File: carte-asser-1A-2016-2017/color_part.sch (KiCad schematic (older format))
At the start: 16 parts, among them P22 CONN_01X02, P23 CONN_01X02, P24 CONN_01X02, U10 OP275, U11 OP275

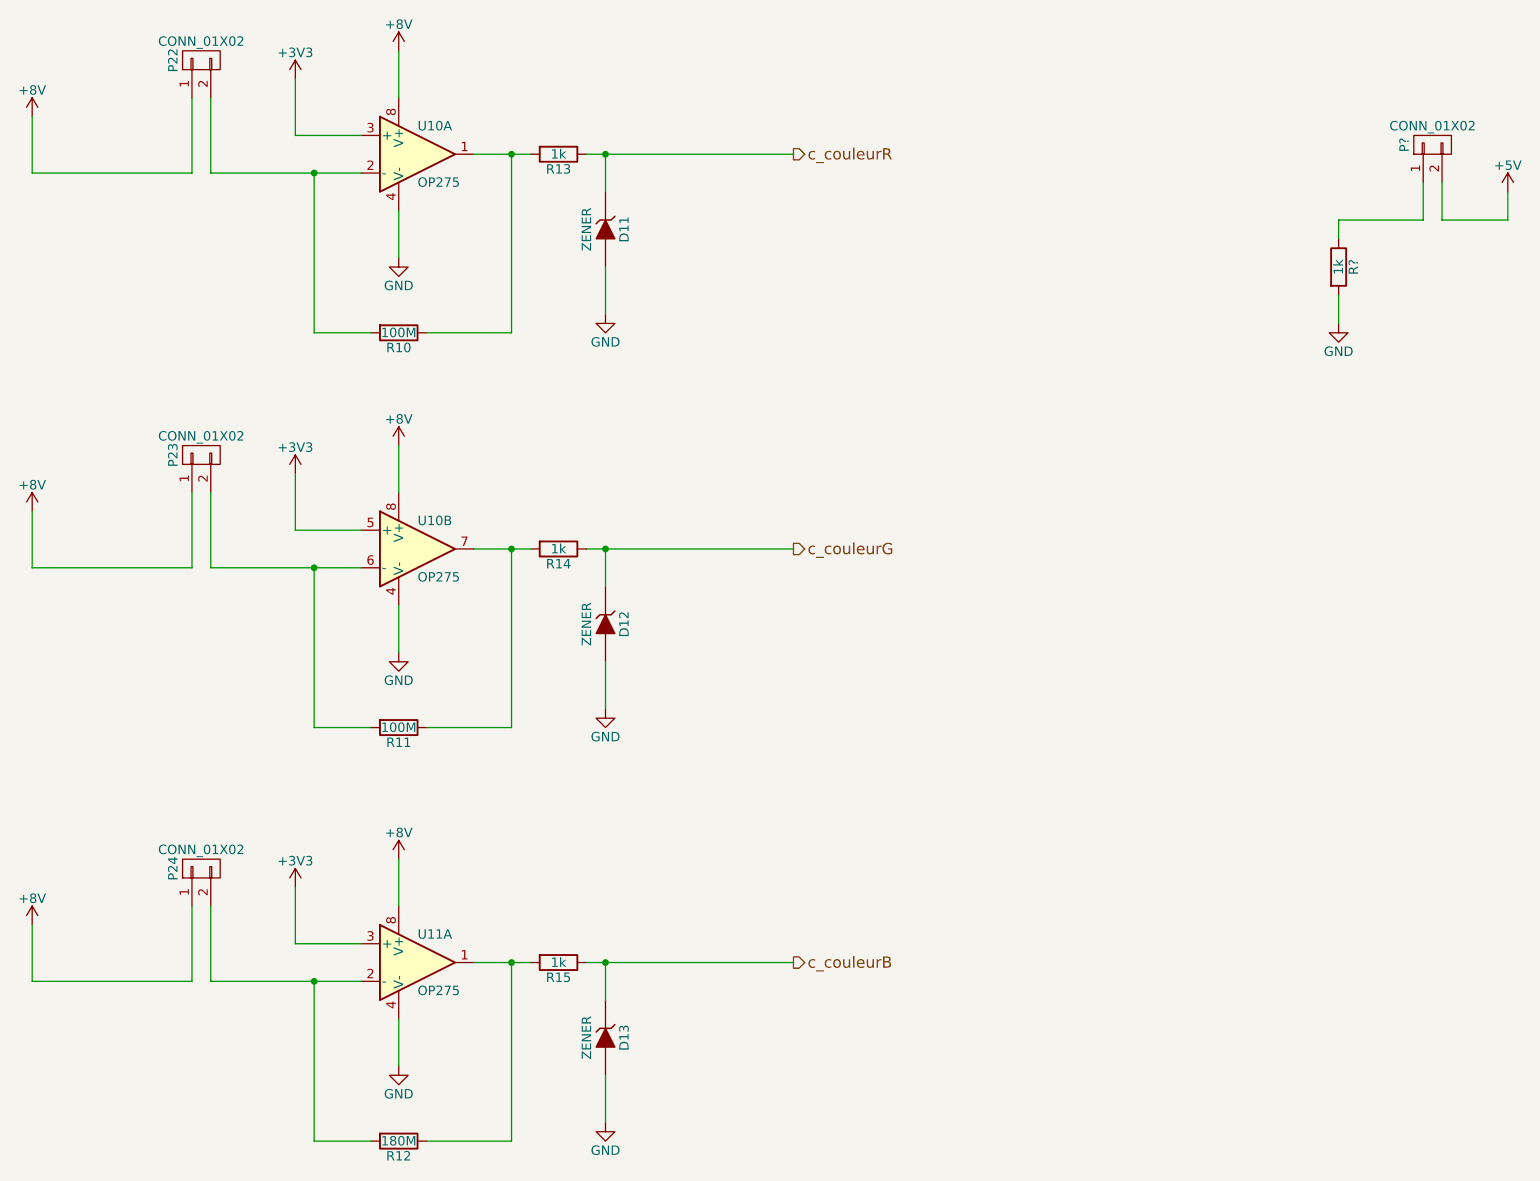
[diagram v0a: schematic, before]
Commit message: PCB
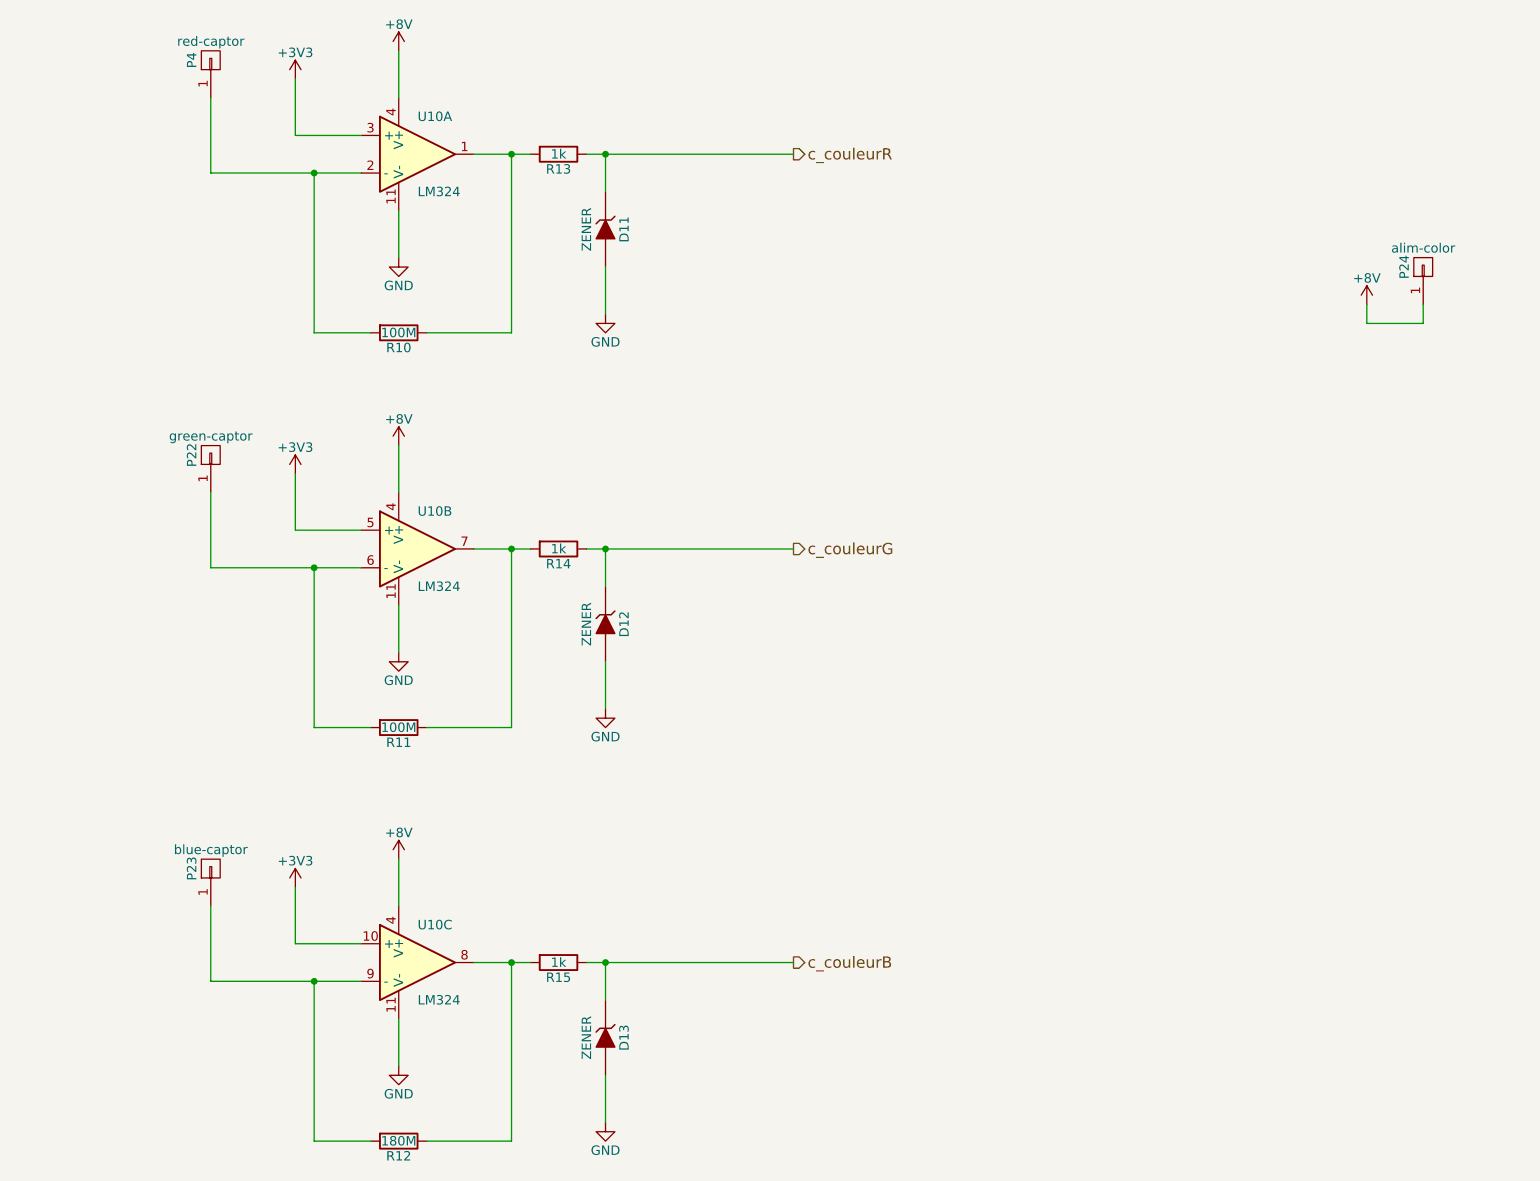
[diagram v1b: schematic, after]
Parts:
- removed P22, P23, P24, P?: CONN_01X02, symbol CONN_01X02
- removed R?: 1k, symbol R
- removed U10, U11: OP275, symbol OP275
- added P22: green-captor, Pin_Headers:Pin_Header_Straight_1x01_Pitch2.54mm, symbol CONN_01X01
- added P23: blue-captor, Pin_Headers:Pin_Header_Straight_1x01_Pitch2.54mm, symbol CONN_01X01
- added P24: alim-color, Pin_Headers:Pin_Header_Straight_1x01_Pitch2.54mm, symbol CONN_01X01
- added P4: red-captor, Pin_Headers:Pin_Header_Straight_1x01_Pitch2.54mm, symbol CONN_01X01
- added U10: LM324, Housings_DIP:DIP-16_W7.62mm, symbol LM324
- D11, D12, D13, R10, R11, R12, R13, R14, R15: footprint (none) -> Discret:R4-LARGE_PADS
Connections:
- net +3V3: now also U10.10 (+), U10.3 (+), U10.5 (+)
- net +8V: now also P24.1 (P1), U10.4 (V+), U10.4 (V+), U10.4 (V+)
- net GND: now also U10.11 (V-), U10.11 (V-), U10.11 (V-)
- net at R10.2: now also P4.1 (P1), U10.2 (-)
- net at R10.1, R13.2: now also U10.1
- net at R11.2: now also P22.1 (P1), U10.6 (-)
- net at R11.1, R14.2: now also U10.7
- net at R12.2: now also P23.1 (P1), U10.9 (-)
- net at R12.1, R15.2: now also U10.8
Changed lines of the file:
@@
 $Descr A4 11693 8268
 encoding utf-8
-Sheet 6 8
+Sheet 6 9
 Title ""
 Date ""
@@
 Comment4 ""
 $EndDescr
-$Comp
-L CONN_01X02 P22
-U 1 1 58A6B5A3
-P 2800 1250
-F 0 "P22" H 2800 1400 50  0000 C CNN
-F 1 "CONN_01X02" V 2900 1250 50  0000 C CNN
-F 2 "" H 2800 1250 50  0000 C CNN
-F 3 "" H 2800 1250 50  0000 C CNN
-	1    2800 1250
-	0    -1   -1   0
-$EndComp
-Wire Wire Line
-	2750 1450 2750 1850
-Wire Wire Line
-	2750 1850 1900 1850
 Wire Wire Line
 	2850 1450 2850 1850
 Wire Wire Line
 	2850 1850 3650 1850
-$Comp
-L OP275 U10
-U 1 1 58A6B640
-P 3950 1750
-F 0 "U10" H 3950 1900 50  0000 L CNN
-F 1 "OP275" H 3950 1600 50  0000 L CNN
-F 2 "" H 3850 1800 50  0000 C CNN
-F 3 "" H 3950 1900 50  0000 C CNN
-	1    3950 1750
-	1    0    0    -1
-$EndComp
 Wire Wire Line
 	3400 1850 3400 2700
@@
 F 0 "R10" V 3930 2700 50  0000 C CNN
 F 1 "100M" V 3850 2700 50  0000 C CNN
-F 2 "" V 3780 2700 50  0000 C CNN
+F 2 "Discret:R4-LARGE_PADS" V 3780 2700 50  0001 C CNN
 F 3 "" H 3850 2700 50  0000 C CNN
 	1    3850 2700
@@
 F 0 "D11" H 4950 2250 50  0000 C CNN
 F 1 "ZENER" H 4950 2050 50  0000 C CNN
-F 2 "" H 4950 2150 50  0000 C CNN
+F 2 "Discret:R4-LARGE_PADS" H 4950 2150 50  0001 C CNN
 F 3 "" H 4950 2150 50  0000 C CNN
 	1    4950 2150
@@
 	3850 1450 3850 1200
 Wire Wire Line
-	1900 1850 1900 1550
-$Comp
-L CONN_01X02 P23
-U 1 1 58A72BC5
-P 2800 3350
-F 0 "P23" H 2800 3500 50  0000 C CNN
-F 1 "CONN_01X02" V 2900 3350 50  0000 C CNN
-F 2 "" H 2800 3350 50  0000 C CNN
-F 3 "" H 2800 3350 50  0000 C CNN
-	1    2800 3350
-	0    -1   -1   0
-$EndComp
-Wire Wire Line
-	2750 3550 2750 3950
-Wire Wire Line
-	2750 3950 1900 3950
-Wire Wire Line
 	2850 3550 2850 3950
 Wire Wire Line
 	2850 3950 3650 3950
-$Comp
-L OP275 U10
-U 2 1 58A72BCF
-P 3950 3850
-F 0 "U10" H 3950 4000 50  0000 L CNN
-F 1 "OP275" H 3950 3700 50  0000 L CNN
-F 2 "" H 3850 3900 50  0000 C CNN
-F 3 "" H 3950 4000 50  0000 C CNN
-	2    3950 3850
-	1    0    0    -1
-$EndComp
 Wire Wire Line
 	3400 3950 3400 4800
@@
 F 0 "R11" V 3930 4800 50  0000 C CNN
 F 1 "100M" V 3850 4800 50  0000 C CNN
-F 2 "" V 3780 4800 50  0000 C CNN
+F 2 "Discret:R4-LARGE_PADS" V 3780 4800 50  0001 C CNN
 F 3 "" H 3850 4800 50  0000 C CNN
 	1    3850 4800
@@
 F 0 "D12" H 4950 4350 50  0000 C CNN
 F 1 "ZENER" H 4950 4150 50  0000 C CNN
-F 2 "" H 4950 4250 50  0000 C CNN
+F 2 "Discret:R4-LARGE_PADS" H 4950 4250 50  0001 C CNN
 F 3 "" H 4950 4250 50  0000 C CNN
 	1    4950 4250
@@
 	3850 3550 3850 3300
 Wire Wire Line
-	1900 3950 1900 3650
-$Comp
-L CONN_01X02 P24
-U 1 1 58A72E17
-P 2800 5550
-F 0 "P24" H 2800 5700 50  0000 C CNN
-F 1 "CONN_01X02" V 2900 5550 50  0000 C CNN
-F 2 "" H 2800 5550 50  0000 C CNN
-F 3 "" H 2800 5550 50  0000 C CNN
-	1    2800 5550
-	0    -1   -1   0
-$EndComp
-Wire Wire Line
-	2750 5750 2750 6150
-Wire Wire Line
-	2750 6150 1900 6150
-Wire Wire Line
 	2850 5750 2850 6150
 Wire Wire Line
 	2850 6150 3650 6150
-$Comp
-L OP275 U11
-U 1 1 58A72E21
-P 3950 6050
-F 0 "U11" H 3950 6200 50  0000 L CNN
-F 1 "OP275" H 3950 5900 50  0000 L CNN
-F 2 "" H 3850 6100 50  0000 C CNN
-F 3 "" H 3950 6200 50  0000 C CNN
-	1    3950 6050
-	1    0    0    -1
-$EndComp
 Wire Wire Line
 	3400 6150 3400 7000
@@
 F 0 "R12" V 3930 7000 50  0000 C CNN
 F 1 "180M" V 3850 7000 50  0000 C CNN
-F 2 "" V 3780 7000 50  0000 C CNN
+F 2 "Discret:R4-LARGE_PADS" V 3780 7000 50  0001 C CNN
 F 3 "" H 3850 7000 50  0000 C CNN
 	1    3850 7000
@@
 F 0 "D13" H 4950 6550 50  0000 C CNN
 F 1 "ZENER" H 4950 6350 50  0000 C CNN
-F 2 "" H 4950 6450 50  0000 C CNN
+F 2 "Discret:R4-LARGE_PADS" H 4950 6450 50  0001 C CNN
 F 3 "" H 4950 6450 50  0000 C CNN
 	1    4950 6450
@@
 Wire Wire Line
 	3850 5750 3850 5500
-Wire Wire Line
-	1900 6150 1900 5850
 $Comp
 L +8V #PWR061
@@
 L +8V #PWR062
 U 1 1 58A7EE3E
-P 1900 1550
-F 0 "#PWR062" H 1900 1400 50  0001 C CNN
-F 1 "+8V" H 1900 1690 50  0000 C CNN
-F 2 "" H 1900 1550 50  0000 C CNN
-F 3 "" H 1900 1550 50  0000 C CNN
-	1    1900 1550
+P 9000 2550
+F 0 "#PWR062" H 9000 2400 50  0001 C CNN
+F 1 "+8V" H 9000 2690 50  0000 C CNN
+F 2 "" H 9000 2550 50  0000 C CNN
+F 3 "" H 9000 2550 50  0000 C CNN
+	1    9000 2550
 	1    0    0    -1
 $EndComp
 $Comp
 L +8V #PWR063
-U 1 1 58A7EF37
-P 1900 3650
-F 0 "#PWR063" H 1900 3500 50  0001 C CNN
-F 1 "+8V" H 1900 3790 50  0000 C CNN
-F 2 "" H 1900 3650 50  0000 C CNN
-F 3 "" H 1900 3650 50  0000 C CNN
-	1    1900 3650
-	1    0    0    -1
-$EndComp
-$Comp
-L +8V #PWR064
 U 1 1 58A7EFDC
 P 3850 3300
-F 0 "#PWR064" H 3850 3150 50  0001 C CNN
+F 0 "#PWR063" H 3850 3150 50  0001 C CNN
 F 1 "+8V" H 3850 3440 50  0000 C CNN
 F 2 "" H 3850 3300 50  0000 C CNN
@@
 $EndComp
 $Comp
-L +8V #PWR065
-U 1 1 58A7F1A1
-P 1900 5850
-F 0 "#PWR065" H 1900 5700 50  0001 C CNN
-F 1 "+8V" H 1900 5990 50  0000 C CNN
-F 2 "" H 1900 5850 50  0000 C CNN
-F 3 "" H 1900 5850 50  0000 C CNN
-	1    1900 5850
-	1    0    0    -1
-$EndComp
-$Comp
-L +8V #PWR066
+L +8V #PWR064
 U 1 1 58A7F216
 P 3850 5500
-F 0 "#PWR066" H 3850 5350 50  0001 C CNN
+F 0 "#PWR064" H 3850 5350 50  0001 C CNN
 F 1 "+8V" H 3850 5640 50  0000 C CNN
 F 2 "" H 3850 5500 50  0000 C CNN
@@
 $EndComp
 $Comp
-L +3V3 #PWR067
+L +3V3 #PWR065
 U 1 1 58A7F34D
 P 3300 5650
-F 0 "#PWR067" H 3300 5500 50  0001 C CNN
+F 0 "#PWR065" H 3300 5500 50  0001 C CNN
 F 1 "+3V3" H 3300 5790 50  0000 C CNN
 F 2 "" H 3300 5650 50  0000 C CNN
@@
 $EndComp
 $Comp
-L +3V3 #PWR068
+L +3V3 #PWR066
 U 1 1 58A7F40A
 P 3300 3450
-F 0 "#PWR068" H 3300 3300 50  0001 C CNN
+F 0 "#PWR066" H 3300 3300 50  0001 C CNN
 F 1 "+3V3" H 3300 3590 50  0000 C CNN
 F 2 "" H 3300 3450 50  0000 C CNN
@@
 $EndComp
 $Comp
-L +3V3 #PWR069
+L +3V3 #PWR067
 U 1 1 58A7F4D3
 P 3300 1350
-F 0 "#PWR069" H 3300 1200 50  0001 C CNN
+F 0 "#PWR067" H 3300 1200 50  0001 C CNN
 F 1 "+3V3" H 3300 1490 50  0000 C CNN
 F 2 "" H 3300 1350 50  0000 C CNN
@@
 F 0 "R13" V 4780 1750 50  0000 C CNN
 F 1 "1k" V 4700 1750 50  0000 C CNN
-F 2 "" V 4630 1750 50  0000 C CNN
+F 2 "Discret:R4-LARGE_PADS" V 4630 1750 50  0001 C CNN
 F 3 "" H 4700 1750 50  0000 C CNN
 	1    4700 1750
@@
 F 0 "R14" V 4780 3850 50  0000 C CNN
 F 1 "1k" V 4700 3850 50  0000 C CNN
-F 2 "" V 4630 3850 50  0000 C CNN
+F 2 "Discret:R4-LARGE_PADS" V 4630 3850 50  0001 C CNN
 F 3 "" H 4700 3850 50  0000 C CNN
 	1    4700 3850
@@
 F 0 "R15" V 4780 6050 50  0000 C CNN
 F 1 "1k" V 4700 6050 50  0000 C CNN
-F 2 "" V 4630 6050 50  0000 C CNN
+F 2 "Discret:R4-LARGE_PADS" V 4630 6050 50  0001 C CNN
 F 3 "" H 4700 6050 50  0000 C CNN
 	1    4700 6050
@@
 	4850 1750 5950 1750
 $Comp
-L CONN_01X02 P?
-U 1 1 58B3D98B
-P 9350 1700
-F 0 "P?" H 9350 1850 50  0000 C CNN
-F 1 "CONN_01X02" V 9450 1700 50  0000 C CNN
-F 2 "" H 9350 1700 50  0000 C CNN
-F 3 "" H 9350 1700 50  0000 C CNN
-	1    9350 1700
+L CONN_01X01 P4
+U 1 1 58BB9EC9
+P 2850 1250
+F 0 "P4" H 2850 1350 50  0000 C CNN
+F 1 "red-captor" V 2950 1250 50  0000 C CNN
+F 2 "Pin_Headers:Pin_Header_Straight_1x01_Pitch2.54mm" H 2850 1250 50  0001 C CNN
+F 3 "" H 2850 1250 50  0000 C CNN
+	1    2850 1250
 	0    -1   -1   0
 $EndComp
-Wire Wire Line
-	9300 1900 9300 2100
-Wire Wire Line
-	9300 2100 8850 2100
-Wire Wire Line
-	8850 2100 8850 2200
-$Comp
-L R R?
-U 1 1 58B3DB16
-P 8850 2350
-F 0 "R?" V 8930 2350 50  0000 C CNN
-F 1 "1k" V 8850 2350 50  0000 C CNN
-F 2 "" V 8780 2350 50  0000 C CNN
-F 3 "" H 8850 2350 50  0000 C CNN
-	1    8850 2350
-	1    0    0    -1
-$EndComp
-Wire Wire Line
-	8850 2500 8850 2650
-$Comp
-L GND #PWR070
-U 1 1 58B3DBAA
-P 8850 2650
-F 0 "#PWR070" H 8850 2400 50  0001 C CNN
-F 1 "GND" H 8850 2500 50  0000 C CNN
-F 2 "" H 8850 2650 50  0000 C CNN
-F 3 "" H 8850 2650 50  0000 C CNN
-	1    8850 2650
-	1    0    0    -1
-$EndComp
-Wire Wire Line
-	9400 1900 9400 2100
-Wire Wire Line
-	9400 2100 9750 2100
-Wire Wire Line
-	9750 2100 9750 1950
-$Comp
-L +5V #PWR071
-U 1 1 58B3DC7A
-P 9750 1950
-F 0 "#PWR071" H 9750 1800 50  0001 C CNN
-F 1 "+5V" H 9750 2090 50  0000 C CNN
-F 2 "" H 9750 1950 50  0000 C CNN
-F 3 "" H 9750 1950 50  0000 C CNN
-	1    9750 1950
-	1    0    0    -1
-$EndComp
+$Comp
+L CONN_01X01 P24
+U 1 1 58BB9FC6
+P 9300 2350
+F 0 "P24" H 9300 2450 50  0000 C CNN
+F 1 "alim-color" V 9400 2350 50  0000 C CNN
+F 2 "Pin_Headers:Pin_Header_Straight_1x01_Pitch2.54mm" H 9300 2350 50  0001 C CNN
+F 3 "" H 9300 2350 50  0000 C CNN
+	1    9300 2350
+	0    -1   -1   0
+$EndComp
+Wire Wire Line
+	9000 2650 9300 2650
+Wire Wire Line
+	9300 2650 9300 2550
+$Comp
+L CONN_01X01 P22
+U 1 1 58BBA20A
+P 2850 3350
+F 0 "P22" H 2850 3450 50  0000 C CNN
+F 1 "green-captor" V 2950 3350 50  0000 C CNN
+F 2 "Pin_Headers:Pin_Header_Straight_1x01_Pitch2.54mm" H 2850 3350 50  0001 C CNN
+F 3 "" H 2850 3350 50  0000 C CNN
+	1    2850 3350
+	0    -1   -1   0
+$EndComp
+$Comp
+L CONN_01X01 P23
+U 1 1 58BBA3AD
+P 2850 5550
+F 0 "P23" H 2850 5650 50  0000 C CNN
+F 1 "blue-captor" V 2950 5550 50  0000 C CNN
+F 2 "Pin_Headers:Pin_Header_Straight_1x01_Pitch2.54mm" H 2850 5550 50  0001 C CNN
+F 3 "" H 2850 5550 50  0000 C CNN
+	1    2850 5550
+	0    -1   -1   0
+$EndComp
+Wire Wire Line
+	9000 2550 9000 2650
+$Comp
+L LM324 U10
+U 1 1 58BCF427
+P 3950 1750
+F 0 "U10" H 3950 1950 50  0000 L CNN
+F 1 "LM324" H 3950 1550 50  0000 L CNN
+F 2 "Housings_DIP:DIP-16_W7.62mm" H 3900 1850 50  0001 C CNN
+F 3 "" H 4000 1950 50  0000 C CNN
+	1    3950 1750
+	1    0    0    -1
+$EndComp
+$Comp
+L LM324 U10
+U 2 1 58BCFA8D
+P 3950 3850
+F 0 "U10" H 3950 4050 50  0000 L CNN
+F 1 "LM324" H 3950 3650 50  0000 L CNN
+F 2 "Housings_DIP:DIP-16_W7.62mm" H 3900 3950 50  0001 C CNN
+F 3 "" H 4000 4050 50  0000 C CNN
+	2    3950 3850
+	1    0    0    -1
+$EndComp
+$Comp
+L LM324 U10
+U 3 1 58BCFB3A
+P 3950 6050
+F 0 "U10" H 3950 6250 50  0000 L CNN
+F 1 "LM324" H 3950 5850 50  0000 L CNN
+F 2 "Housings_DIP:DIP-16_W7.62mm" H 3900 6150 50  0001 C CNN
+F 3 "" H 4000 6250 50  0000 C CNN
+	3    3950 6050
+	1    0    0    -1
+$EndComp
